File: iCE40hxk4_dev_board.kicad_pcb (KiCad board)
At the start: 4 copper layers, 141 parts, among them J201 CONN_01X02, J202 USB_OTG, J401 CONN_01X35, J501 CONN_01X35, U201 MIC2005A-2, U203 93LCxxB_sot-23-6, U204 MIC5355/6-xYMME, U205 FT2232H, U301 iCE40-HX4K-TQ144, U302 25LC_EEPROM, U501 AS4C1M16S

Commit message: Continued with routing...
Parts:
- C201: moved to F.Cu
- C220, C221, C222, C223, C224, C315, C501, C504, C505, L203, R301, R302, R307, R401, R402, R403, R404, R405, R406, R407, R408: moved to B.Cu
- moved C407 187.8 mm to (199.0, 91.9), turned to 90 degrees
- moved R402 160.5 mm to (194.6, 103.4)
- moved R307 160.2 mm to (175.5, 103.4)
- moved C503 151.3 mm to (148.3, 107.4), turned to 270 degrees
- moved R404 151.1 mm to (194.7, 100.8)
- moved R308 146.5 mm to (181.6, 79.5), turned to 180 degrees
- moved C508 144.1 mm to (148.3, 102.7), turned to 270 degrees
- moved C501 136.6 mm to (166.5, 102.2), turned to 270 degrees
- moved R405 123.5 mm to (194.7, 99.7)
- moved C316 120.7 mm to (177.4, 82.9), turned to 180 degrees
- moved R406 115.6 mm to (194.7, 98.6)
- moved D301 109.2 mm to (192.9, 83.5), turned to 180 degrees
- moved C317 104.7 mm to (178.6, 81.2), turned to 180 degrees
- moved D401 104.1 mm to (194.7, 104.6)
- moved C507 103.3 mm to (160.0, 91.2), turned to 180 degrees
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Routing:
- net +3V3: track 41.9 -> 79.5 mm, vias 6 -> 18
- net GND: track 29.6 -> 50.7 mm, vias 21 -> 24
- net Net-(C213-Pad1): track 14.2 -> 3.46 mm, vias 2 -> 1
- net Net-(C314-Pad1): track 0.00 -> 8.40 mm, vias 0 -> 1
- net Net-(C316-Pad1): track 0.00 -> 7.78 mm
- net /RIGHT_TOP_BANKs/IOR_117: track 0.00 -> 7.67 mm
- net /RIGHT_TOP_BANKs/IOR_116: track 0.00 -> 7.35 mm
- net /RIGHT_TOP_BANKs/IOR_115: track 0.00 -> 6.98 mm
- net /RIGHT_TOP_BANKs/IOR_114: track 0.00 -> 6.71 mm
- net /RIGHT_TOP_BANKs/IOR_112: track 0.00 -> 6.69 mm
- net /RIGHT_TOP_BANKs/IOR_111: track 0.00 -> 6.33 mm
- net /RIGHT_TOP_BANKs/IOR_109: track 0.00 -> 6.32 mm
- net /RIGHT_TOP_BANKs/IOR_110: track 0.00 -> 6.01 mm
- net Net-(D301-Pad1): track 0.00 -> 5.85 mm
- net Net-(C314-Pad2): track 0.00 -> 4.86 mm, vias 0 -> 1
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- removed copper zone on F.Cu, net +3V3

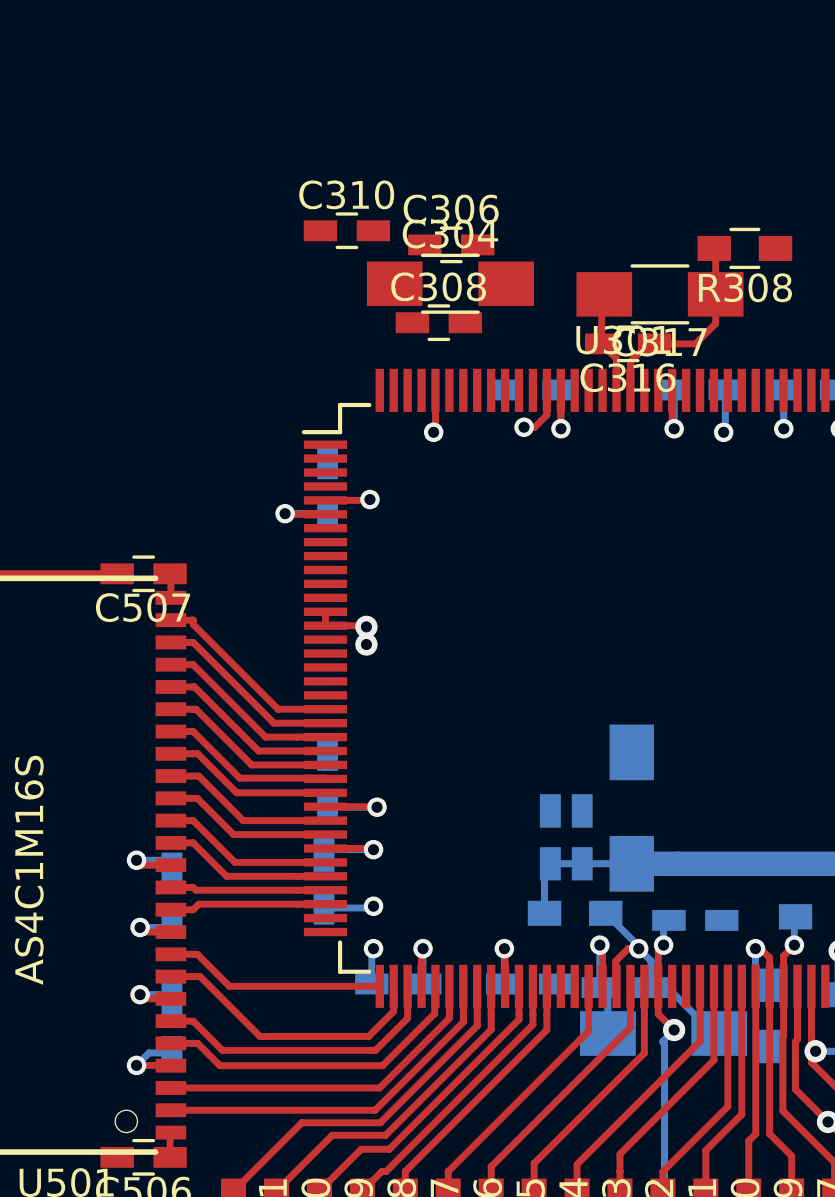
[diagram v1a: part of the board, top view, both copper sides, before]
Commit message: Continued with routing...
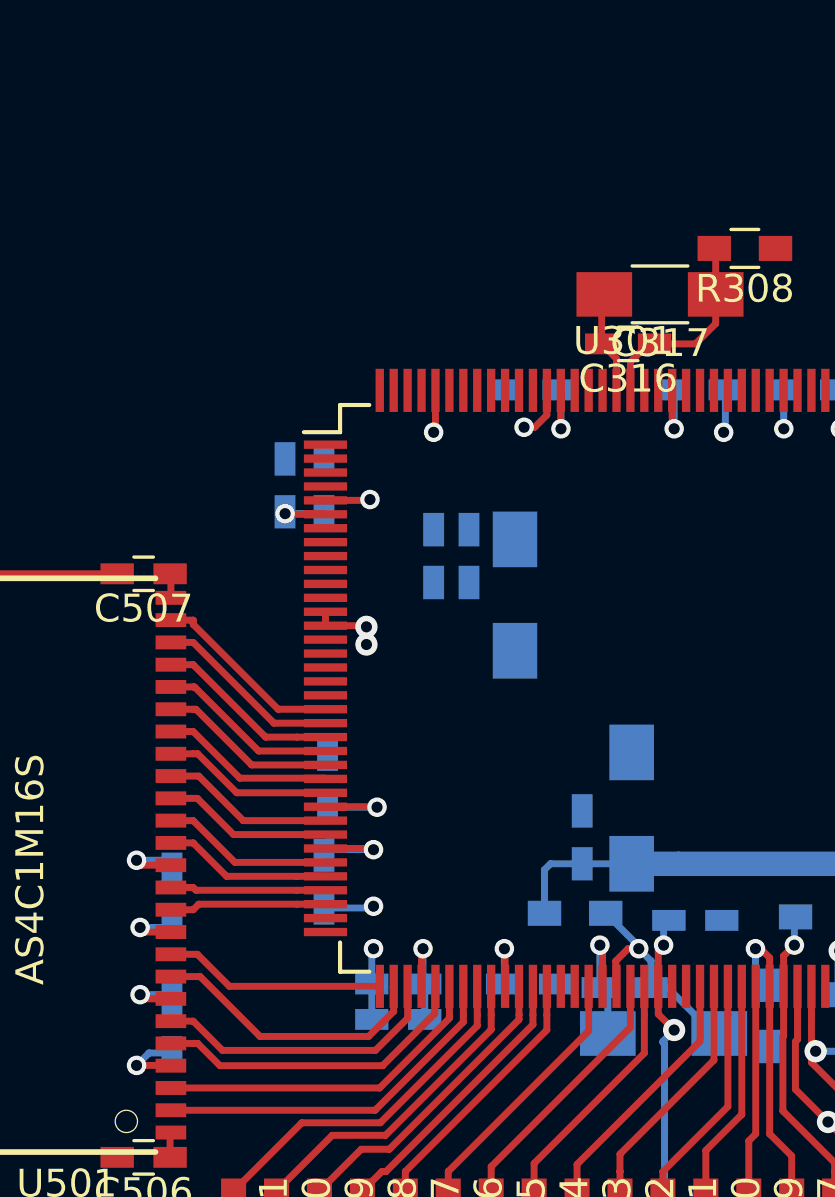
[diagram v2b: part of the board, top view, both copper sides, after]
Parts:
- C304, C306, C308, C310: moved to B.Cu
- moved C304 11.4 mm to (173.4, 91.9), turned to 270 degrees
- moved C306 11.2 mm to (171.7, 90.6), turned to 90 degrees
- moved C310 9.18 mm to (166.5, 88.0), turned to 90 degrees
- moved C308 8.38 mm to (170.4, 90.6), turned to 90 degrees
- moved C312 7.59 mm to (169.2, 105.9), turned to 180 degrees
- moved C502 1.53 mm to (165.1, 88.0)
- moved C311 1.27 mm to (169.2, 107.2)
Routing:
- net GND: track 50.7 -> 51.9 mm
- net /FPGA_PROGRAMMING+POWER/+1.2V: track 64.3 -> 65.6 mm
